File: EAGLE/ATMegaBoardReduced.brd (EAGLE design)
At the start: 57.1 x 50.5 mm, 17 parts, among them IC2 ATMEGA168-20P, IC3 REG1117, X1 49S/18PF

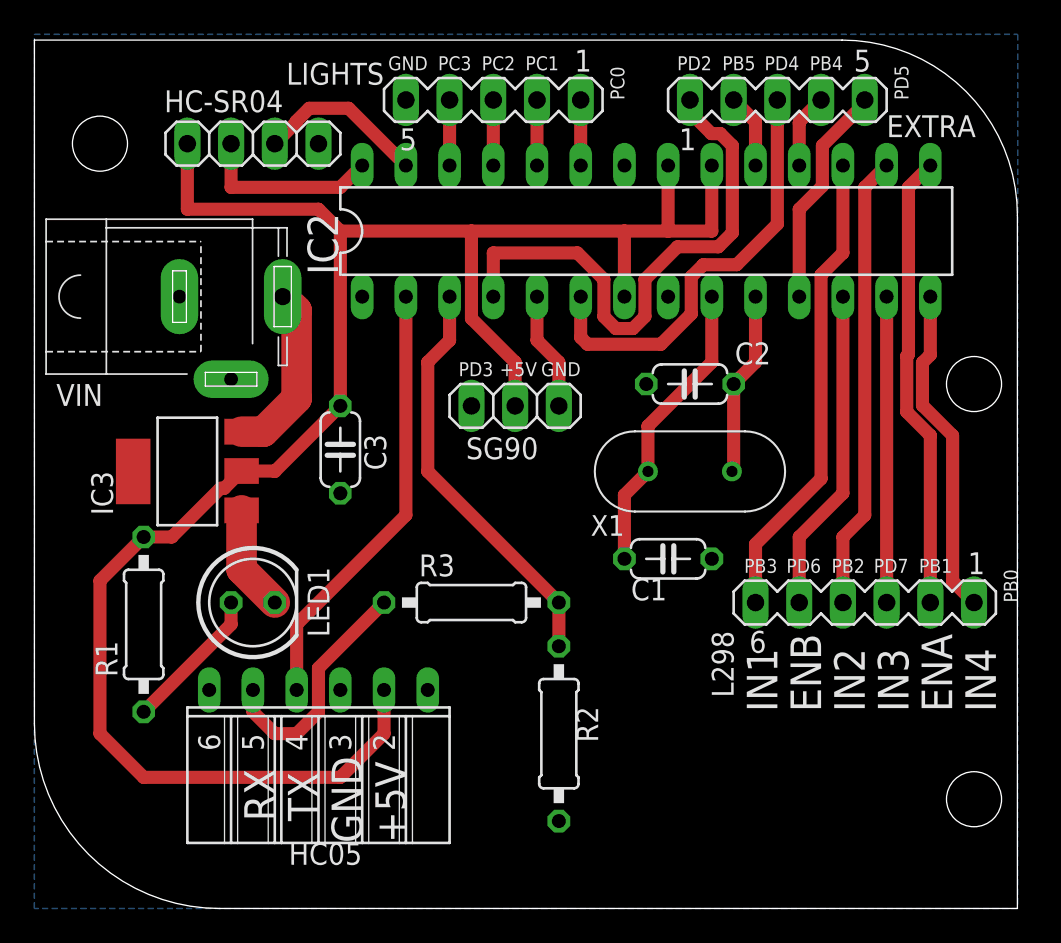
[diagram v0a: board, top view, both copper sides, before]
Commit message: minor layout changes
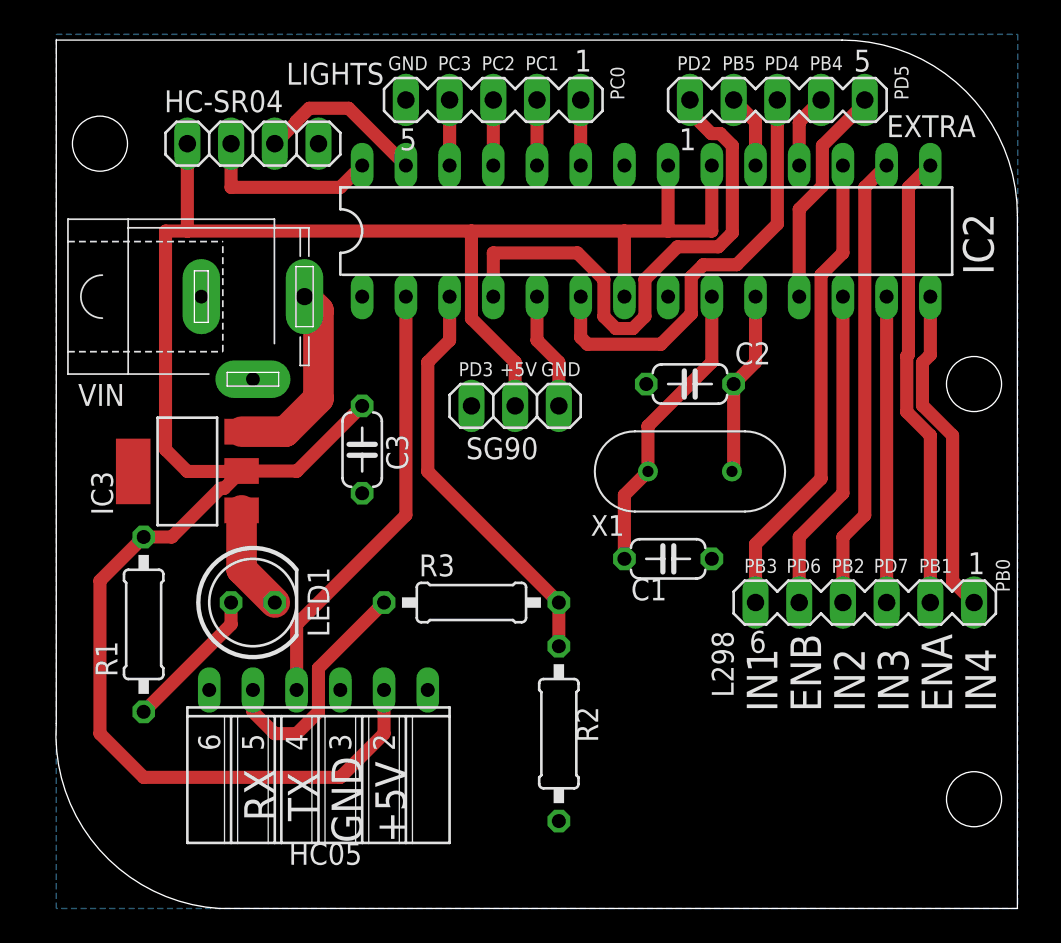
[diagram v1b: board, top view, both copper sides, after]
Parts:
- moved C3 1.27 mm to (30.5, 31.8)
- moved VIN 1.27 mm to (24.1, 40.6)
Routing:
- net +5V: track 115.9 -> 126.7 mm
- net VIN: track 10.3 -> 11.5 mm
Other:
- board size 57.1 x 50.5 mm -> 55.9 x 50.5 mm
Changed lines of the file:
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@@
 <board>
 <plain>
-<wire x1="58.37200625" y1="55.55" x2="11.43" y2="55.55" width="0" layer="20"/>
-<wire x1="11.43" y1="55.55" x2="11.43" y2="15.8294" width="0" layer="20"/>
-<wire x1="11.43" y1="15.8294" x2="22.1794" y2="5.08" width="0" layer="20" curve="90"/>
+<wire x1="58.37200625" y1="55.55" x2="12.7" y2="55.55" width="0" layer="20"/>
+<wire x1="12.7" y1="55.55" x2="12.7" y2="15.8294" width="0" layer="20"/>
+<wire x1="12.7" y1="15.8294" x2="22.1794" y2="5.08" width="0" layer="20" curve="90"/>
 <wire x1="22.1794" y1="5.08" x2="68.56" y2="5.08" width="0" layer="20"/>
 <wire x1="68.56" y1="5.08" x2="68.56" y2="45.36200625" width="0" layer="20"/>
@@
 <text x="62.23" y="25.4" size="0.8128" layer="21" rot="R180">PD7</text>
 <text x="64.77" y="25.4" size="0.8128" layer="21" rot="R180">PB1</text>
-<text x="68.58" y="22.86" size="0.8128" layer="21" rot="R90">PB0</text>
+<text x="67.31" y="25.4" size="0.8128" layer="21" rot="R270">PB0</text>
 </plain>
 <attributes>
@@
 </element>
 <element name="IC2" library="adafruit" package="DIL28-3" value="ATMEGA168-20P" x="46.99" y="44.45" smashed="yes">
-<attribute name="NAME" x="29.083" y="41.91" size="1.778" layer="25" ratio="10" rot="R90"/>
+<attribute name="NAME" x="67.183" y="41.91" size="1.778" layer="25" ratio="10" rot="R90"/>
 <attribute name="VALUE" x="31.242" y="43.5102" size="1.778" layer="27" ratio="10"/>
 </element>
@@
 <attribute name="VALUE" x="26.162" y="27.686" size="1.27" layer="27" ratio="10" rot="R90"/>
 </element>
-<element name="C3" library="rcl" library_urn="urn:adsk.eagle:library:334" package="C050-024X044" package3d_urn="urn:adsk.eagle:package:23643/1" value="220uF" x="29.21" y="31.75" smashed="yes" rot="R270">
-<attribute name="NAME" x="30.607" y="32.639" size="1.27" layer="25" ratio="10" rot="R270"/>
-<attribute name="POPULARITY" value="14" x="29.21" y="31.75" size="1.778" layer="27" rot="R270" display="off"/>
-<attribute name="SPICEPREFIX" value="C" x="29.21" y="31.75" size="1.778" layer="27" rot="R270" display="off"/>
-<attribute name="VALUE" x="26.543" y="33.909" size="1.27" layer="27" ratio="10" rot="R270"/>
+<element name="C3" library="rcl" library_urn="urn:adsk.eagle:library:334" package="C050-024X044" package3d_urn="urn:adsk.eagle:package:23643/1" value="220uF" x="30.48" y="31.75" smashed="yes" rot="R270">
+<attribute name="NAME" x="31.877" y="32.639" size="1.27" layer="25" ratio="10" rot="R270"/>
+<attribute name="POPULARITY" value="14" x="30.48" y="31.75" size="1.778" layer="27" rot="R270" display="off"/>
+<attribute name="SPICEPREFIX" value="C" x="30.48" y="31.75" size="1.778" layer="27" rot="R270" display="off"/>
+<attribute name="VALUE" x="27.813" y="33.909" size="1.27" layer="27" ratio="10" rot="R270"/>
 </element>
 <element name="R1" library="rcl" library_urn="urn:adsk.eagle:library:334" package="0207/10" package3d_urn="urn:adsk.eagle:package:23491/2" value="1k" x="17.78" y="21.59" smashed="yes" rot="R90">
@@
 <attribute name="VALUE" x="27.3304" y="21.0566" size="1.27" layer="27" ratio="10"/>
 </element>
-<element name="VIN" library="con-jack" library_urn="urn:adsk.eagle:library:154" package="SPC4078" package3d_urn="urn:adsk.eagle:package:7494/1" value="" x="22.86" y="40.64" smashed="yes">
-<attribute name="MF" value="" x="22.86" y="40.64" size="1.778" layer="27" display="off"/>
-<attribute name="MPN" value="" x="22.86" y="40.64" size="1.778" layer="27" display="off"/>
-<attribute name="NAME" x="12.7" y="34.29" size="1.27" layer="25"/>
-<attribute name="OC_FARNELL" value="unknown" x="22.86" y="40.64" size="1.778" layer="27" display="off"/>
-<attribute name="OC_NEWARK" value="unknown" x="22.86" y="40.64" size="1.778" layer="27" display="off"/>
-<attribute name="POPULARITY" value="3" x="22.86" y="40.64" size="1.778" layer="27" display="off"/>
-<attribute name="VALUE" x="12.7" y="34.29" size="1.27" layer="27"/>
+<element name="VIN" library="con-jack" library_urn="urn:adsk.eagle:library:154" package="SPC4078" package3d_urn="urn:adsk.eagle:package:7494/1" value="" x="24.13" y="40.64" smashed="yes">
+<attribute name="MF" value="" x="24.13" y="40.64" size="1.778" layer="27" display="off"/>
+<attribute name="MPN" value="" x="24.13" y="40.64" size="1.778" layer="27" display="off"/>
+<attribute name="NAME" x="13.97" y="34.29" size="1.27" layer="25"/>
+<attribute name="OC_FARNELL" value="unknown" x="24.13" y="40.64" size="1.778" layer="27" display="off"/>
+<attribute name="OC_NEWARK" value="unknown" x="24.13" y="40.64" size="1.778" layer="27" display="off"/>
+<attribute name="POPULARITY" value="3" x="24.13" y="40.64" size="1.778" layer="27" display="off"/>
+<attribute name="VALUE" x="13.97" y="34.29" size="1.27" layer="27"/>
 </element>
 <element name="R2" library="rcl" library_urn="urn:adsk.eagle:library:334" package="0207/10" package3d_urn="urn:adsk.eagle:package:23491/2" value="2k" x="41.91" y="15.24" smashed="yes" rot="R90">
@@
 <contactref element="R1" pad="2"/>
 <contactref element="HC05" pad="2"/>
-<wire x1="25.4" y1="30.48" x2="29.21" y2="34.29" width="0.762" layer="1"/>
-<wire x1="29.21" y1="34.29" x2="29.21" y2="44.45" width="0.762" layer="1"/>
-<wire x1="29.21" y1="44.45" x2="36.83" y2="44.45" width="0.762" layer="1"/>
+<wire x1="36.83" y1="44.45" x2="20.32" y2="44.45" width="0.762" layer="1"/>
 <wire x1="36.83" y1="44.45" x2="45.72" y2="44.45" width="0.762" layer="1"/>
 <wire x1="45.72" y1="44.45" x2="48.26" y2="44.45" width="0.762" layer="1"/>
@@
 <wire x1="17.78" y1="12.7" x2="29.21" y2="12.7" width="0.762" layer="1"/>
 <wire x1="31.75" y1="15.24" x2="31.75" y2="17.78" width="0.762" layer="1"/>
-<wire x1="27.94" y1="45.72" x2="20.32" y2="45.72" width="0.762" layer="1"/>
-<wire x1="20.32" y1="45.72" x2="20.32" y2="49.53" width="0.762" layer="1"/>
-<wire x1="29.21" y1="44.45" x2="27.94" y2="45.72" width="0.762" layer="1"/>
 <wire x1="17.78" y1="12.7" x2="15.24" y2="15.24" width="0.762" layer="1"/>
 <wire x1="23.4696" y1="30.5054" x2="22.4663" y2="29.5021" width="0.762" layer="1"/>
@@
 <wire x1="22.24535625" y1="29.5021" x2="19.41325625" y2="26.67" width="0.762" layer="1"/>
 <wire x1="19.41325625" y1="26.67" x2="17.78" y2="26.67" width="0.762" layer="1"/>
-<wire x1="23.4696" y1="30.5054" x2="25.3746" y2="30.5054" width="0.762" layer="1"/>
-<wire x1="25.3746" y1="30.5054" x2="25.4" y2="30.48" width="0.762" layer="1"/>
+<wire x1="23.4696" y1="30.5054" x2="26.6446" y2="30.5054" width="0.762" layer="1"/>
+<wire x1="26.6446" y1="30.5054" x2="26.67" y2="30.48" width="0.762" layer="1"/>
 <wire x1="36.83" y1="44.45" x2="36.83" y2="39.37" width="0.762" layer="1"/>
 <wire x1="39.37" y1="34.29" x2="39.37" y2="36.83" width="0.762" layer="1"/>
 <wire x1="39.37" y1="36.83" x2="36.83" y2="39.37" width="0.762" layer="1"/>
 <wire x1="29.21" y1="12.7" x2="31.75" y2="15.24" width="0.762" layer="1"/>
+<wire x1="26.6446" y1="30.5054" x2="26.6954" y2="30.5054" width="0.762" layer="1"/>
+<wire x1="26.6954" y1="30.5054" x2="30.48" y2="34.29" width="0.762" layer="1"/>
+<wire x1="23.4696" y1="30.5054" x2="23.4442" y2="30.48" width="0.762" layer="1"/>
+<wire x1="23.4442" y1="30.48" x2="20.32" y2="30.48" width="0.762" layer="1"/>
+<wire x1="20.32" y1="30.48" x2="19.05" y2="31.75" width="0.762" layer="1"/>
+<wire x1="19.05" y1="31.75" x2="19.05" y2="44.45" width="0.762" layer="1"/>
+<wire x1="20.32" y1="44.45" x2="19.05" y2="44.45" width="0.762" layer="1"/>
+<wire x1="20.32" y1="49.53" x2="20.32" y2="44.45" width="0.762" layer="1"/>
 </signal>
 <signal name="GND" class="1">
@@
 <contactref element="R2" pad="1"/>
 <polygon width="0.1524" layer="16">
-<vertex x="11.43" y="5.08"/>
-<vertex x="11.43" y="55.88"/>
+<vertex x="12.7" y="5.08"/>
+<vertex x="12.7" y="55.88"/>
 <vertex x="68.58" y="55.88"/>
 <vertex x="68.58" y="5.08"/>
@@
 <contactref element="IC3" pad="3"/>
 <contactref element="VIN" pad="3"/>
-<wire x1="25.86" y1="40.64" x2="26.67" y2="39.83" width="1.778" layer="1"/>
-<wire x1="26.67" y1="34.7218" x2="24.7396" y2="32.7914" width="1.778" layer="1"/>
-<wire x1="24.7396" y1="32.7914" x2="23.4696" y2="32.7914" width="1.778" layer="1"/>
-<wire x1="26.67" y1="39.83" x2="26.67" y2="34.7218" width="1.778" layer="1"/>
+<wire x1="27.94" y1="34.7218" x2="26.0096" y2="32.7914" width="1.778" layer="1"/>
+<wire x1="26.0096" y1="32.7914" x2="23.4696" y2="32.7914" width="1.778" layer="1"/>
+<wire x1="27.13" y1="40.64" x2="27.94" y2="39.83" width="1.778" layer="1"/>
+<wire x1="27.94" y1="39.83" x2="27.94" y2="34.7218" width="1.778" layer="1"/>
 </signal>
 <signal name="IN4">
